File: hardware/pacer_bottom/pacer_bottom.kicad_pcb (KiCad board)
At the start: 2 copper layers, 88.2 x 28.1 mm, 13 parts, among them J1 Conn_01x02_Socket, J2 Conn_01x02_Socket, SW1 SW_SPST

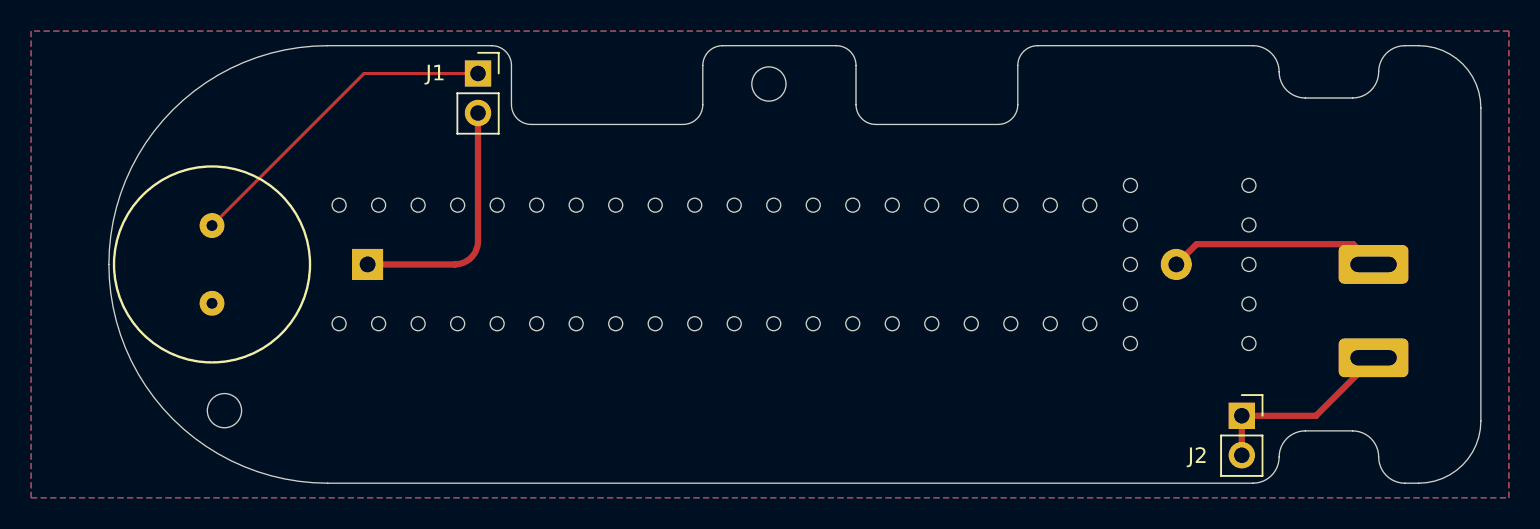
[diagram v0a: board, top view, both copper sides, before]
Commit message: hardware update after prototype
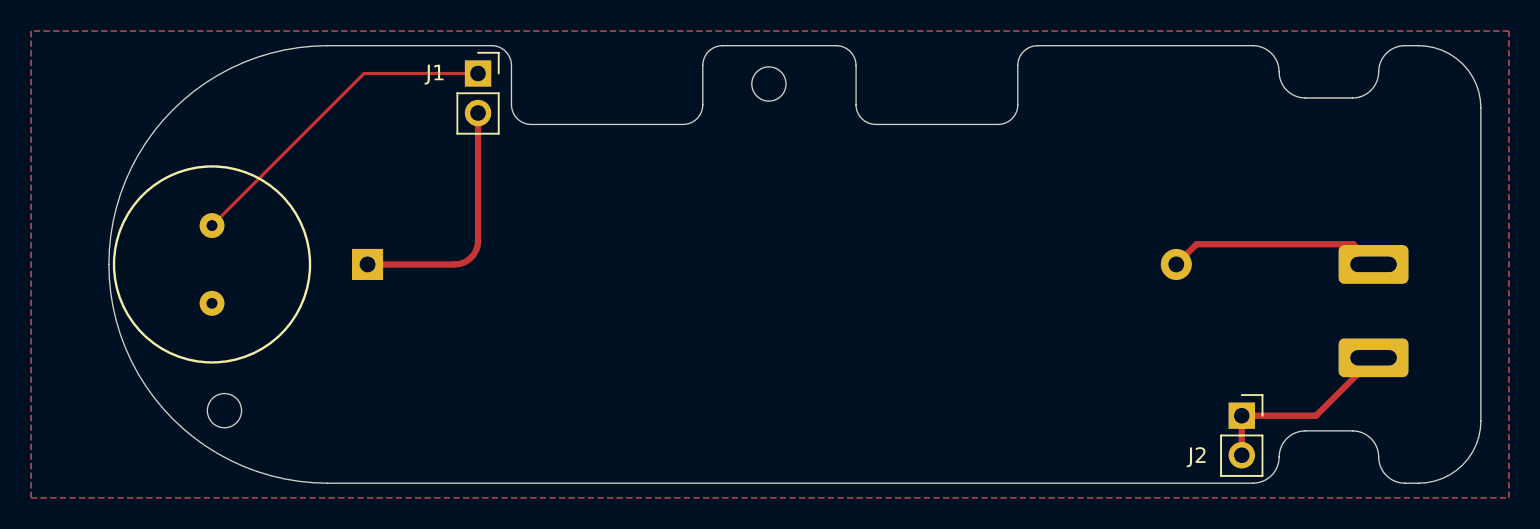
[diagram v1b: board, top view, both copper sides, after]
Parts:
- removed the H1 at (114.8, 103.8)
- removed the H2 at (140.2, 103.8)
- removed H3: MountingHole, My_lib:OSX05201-mount
- renumbered H4 to H1, H5 to H2
